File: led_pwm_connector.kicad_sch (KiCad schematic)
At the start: 7 parts, among them CN7 JST_VH_8PIN_10A_250V

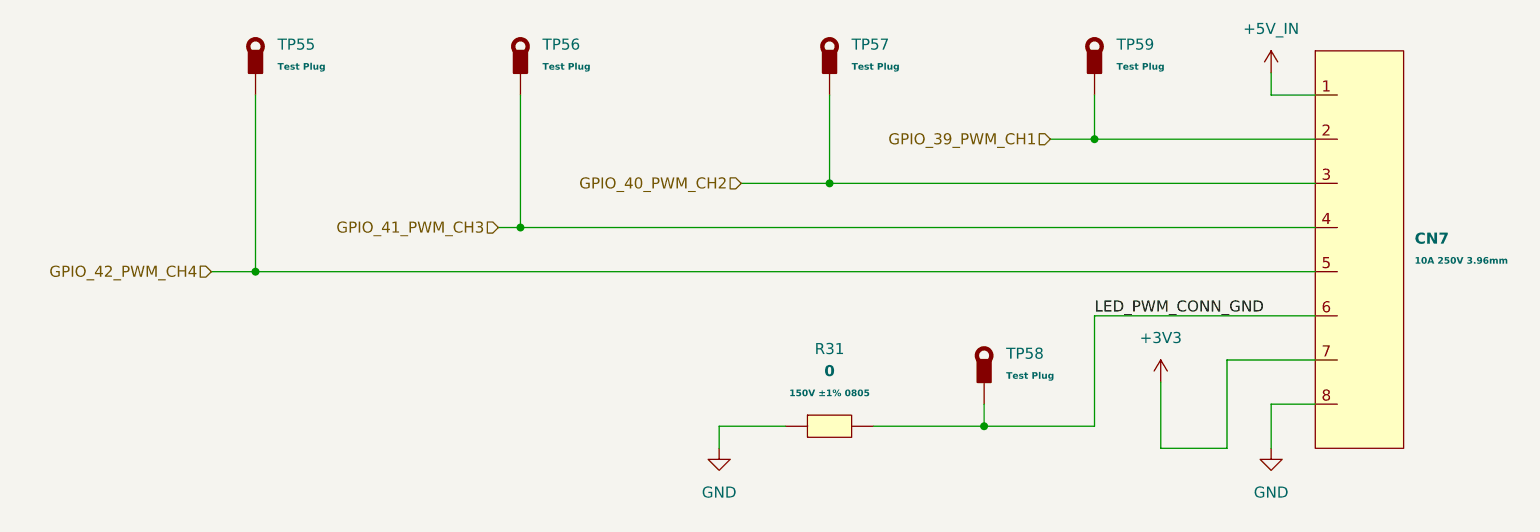
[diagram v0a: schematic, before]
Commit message: commit before updating to LiveAstra lib
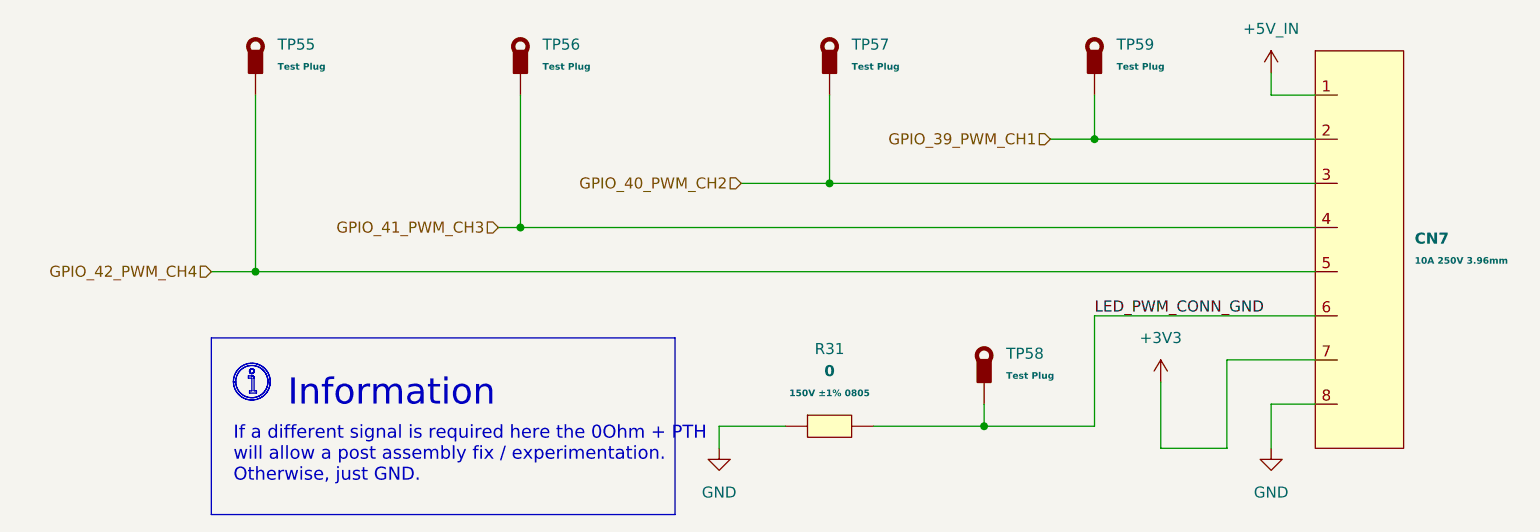
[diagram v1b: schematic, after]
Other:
- note added: "If a different signal is required here the 0Ohm + PTH will allow a post assembly fix / experimentation. Otherwise, just GND."
- note added: "Information"
